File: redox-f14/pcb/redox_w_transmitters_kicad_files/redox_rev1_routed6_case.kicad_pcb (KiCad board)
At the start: 2 copper layers, 166.4 x 135.9 mm, 31 parts, among them K0 KEYSW, K1 KEYSW, K10 KEYSW, K11 KEYSW, K12 KEYSW, K13 KEYSW, K14 KEYSW, K15 KEYSW, K16 KEYSW, K2 KEYSW, K20 KEYSW, K21 KEYSW, K22 KEYSW, K23 KEYSW, K24 KEYSW, K25 KEYSW, K26 KEYSW, K3 KEYSW, K30 KEYSW, K31 KEYSW, K32 KEYSW, K33 KEYSW, K34 KEYSW, K35 KEYSW, K4 KEYSW, K42 KEYSW, K43 KEYSW, K44 KEYSW, K45 KEYSW, K5 KEYSW, K6 KEYSW

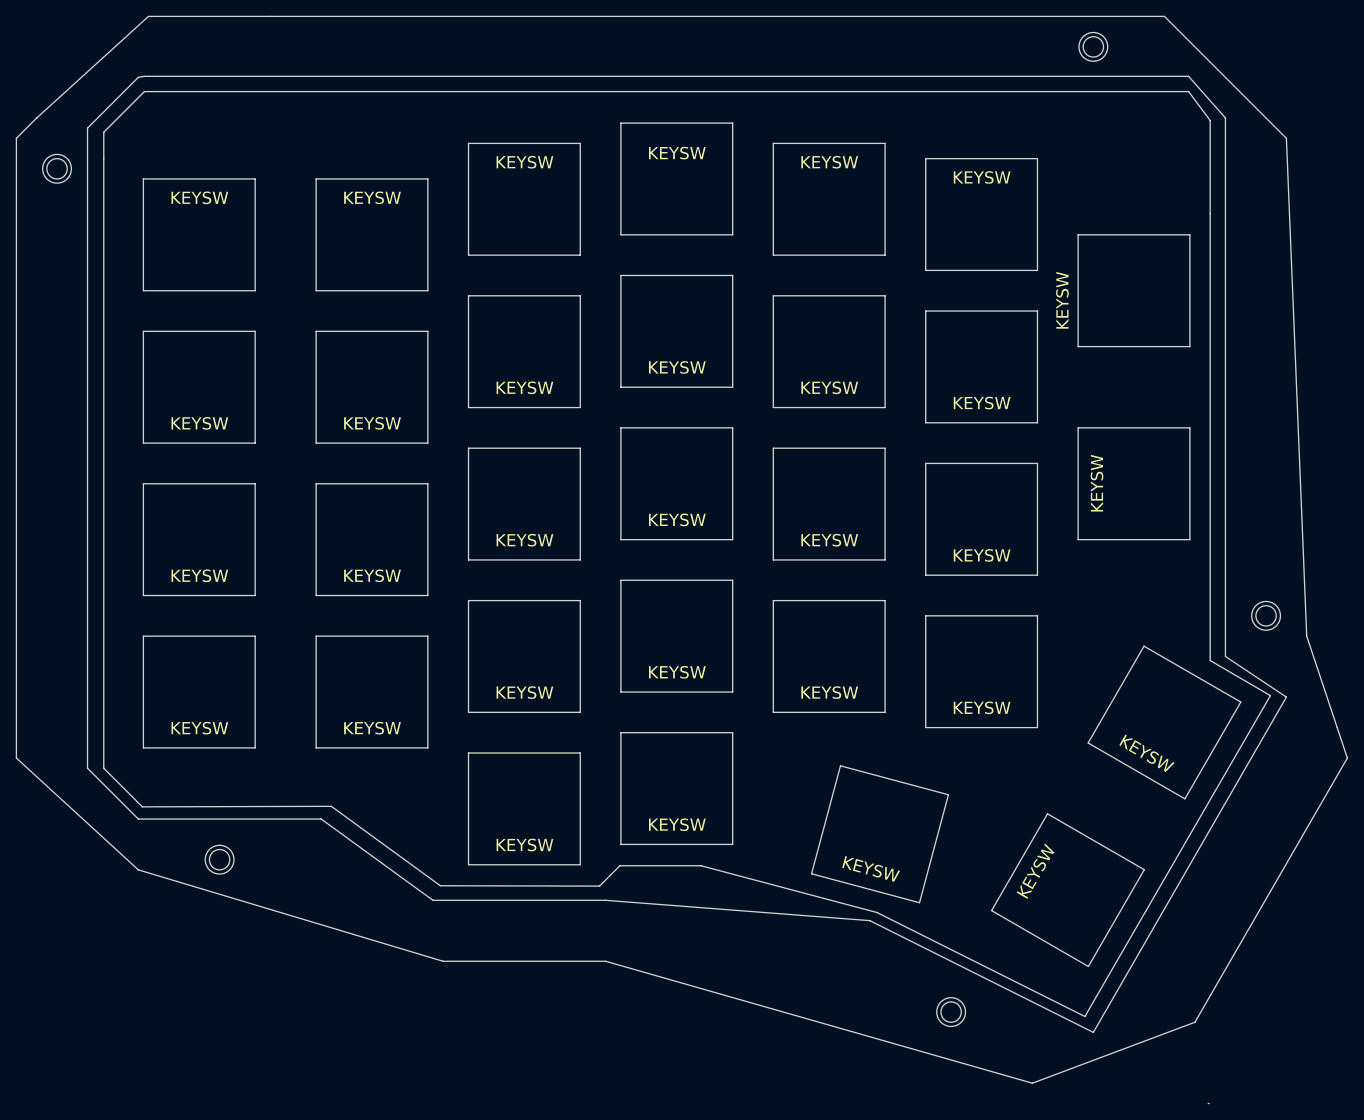
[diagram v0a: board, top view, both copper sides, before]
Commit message: update case v2
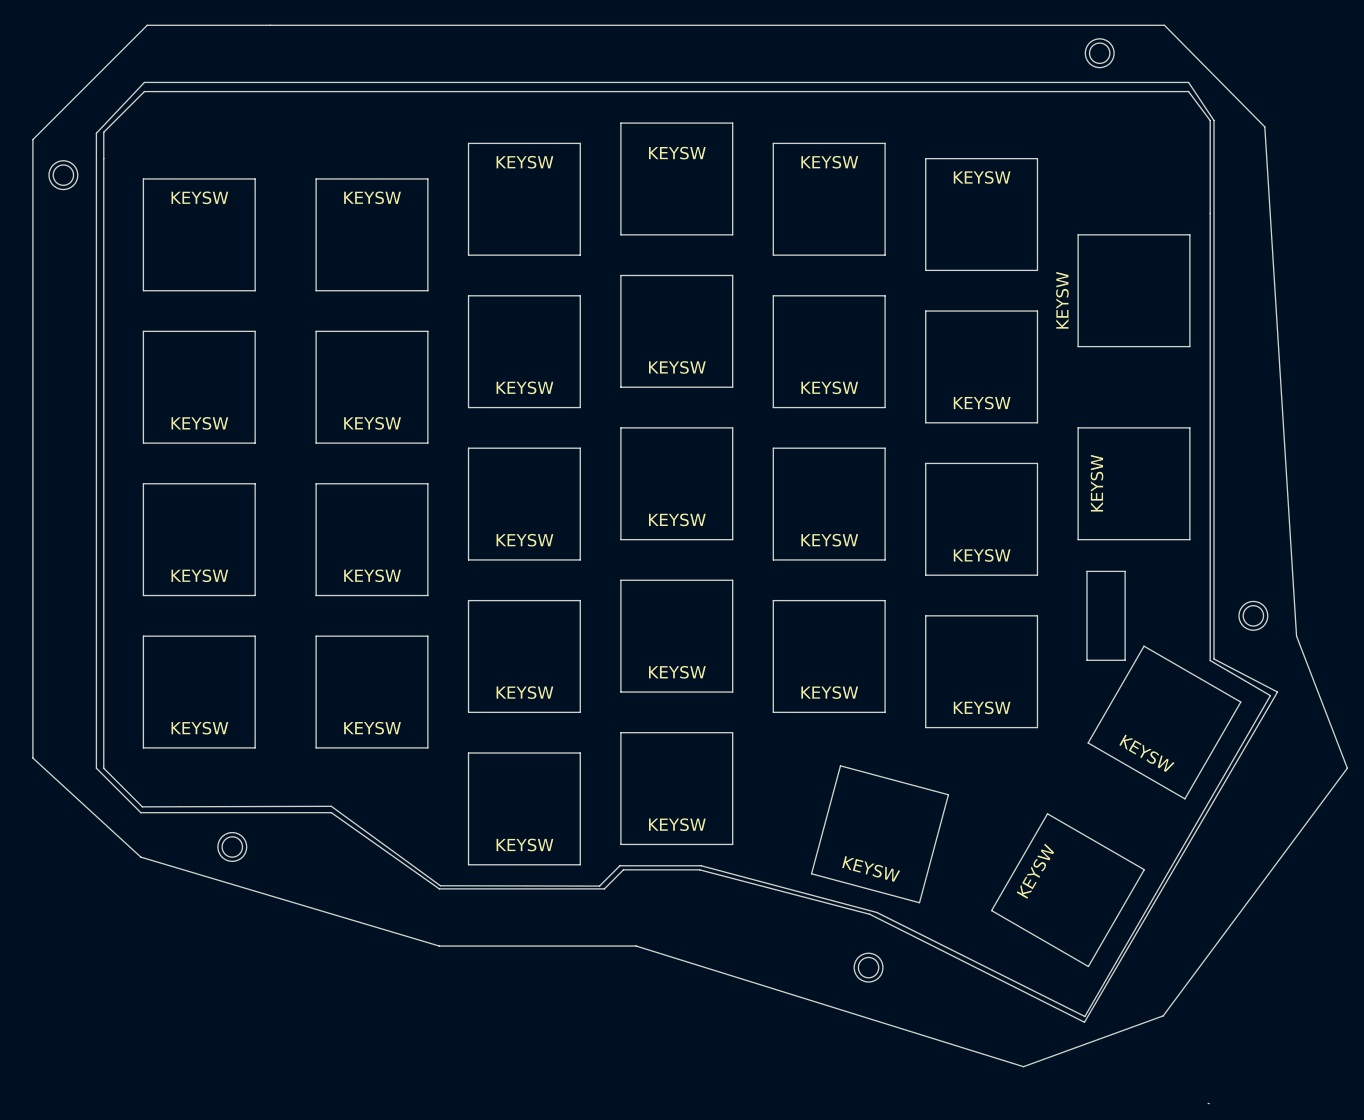
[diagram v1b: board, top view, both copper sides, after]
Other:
- board size 166.4 x 135.9 mm -> 164.3 x 134.8 mm
